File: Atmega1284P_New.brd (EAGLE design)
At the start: 69.5 x 53.3 mm, 28 parts, among them U3 ESP-WROOM-32

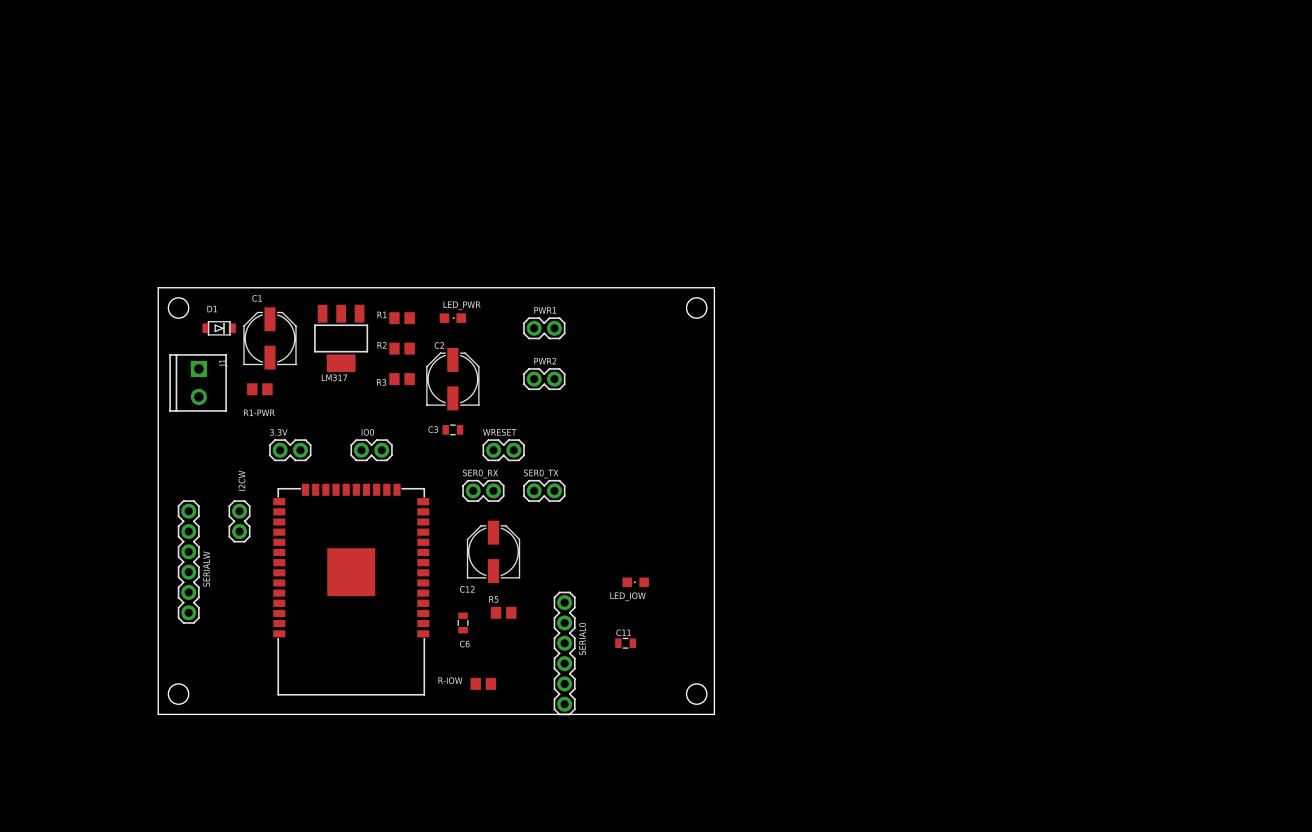
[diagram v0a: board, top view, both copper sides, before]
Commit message: Working Copy
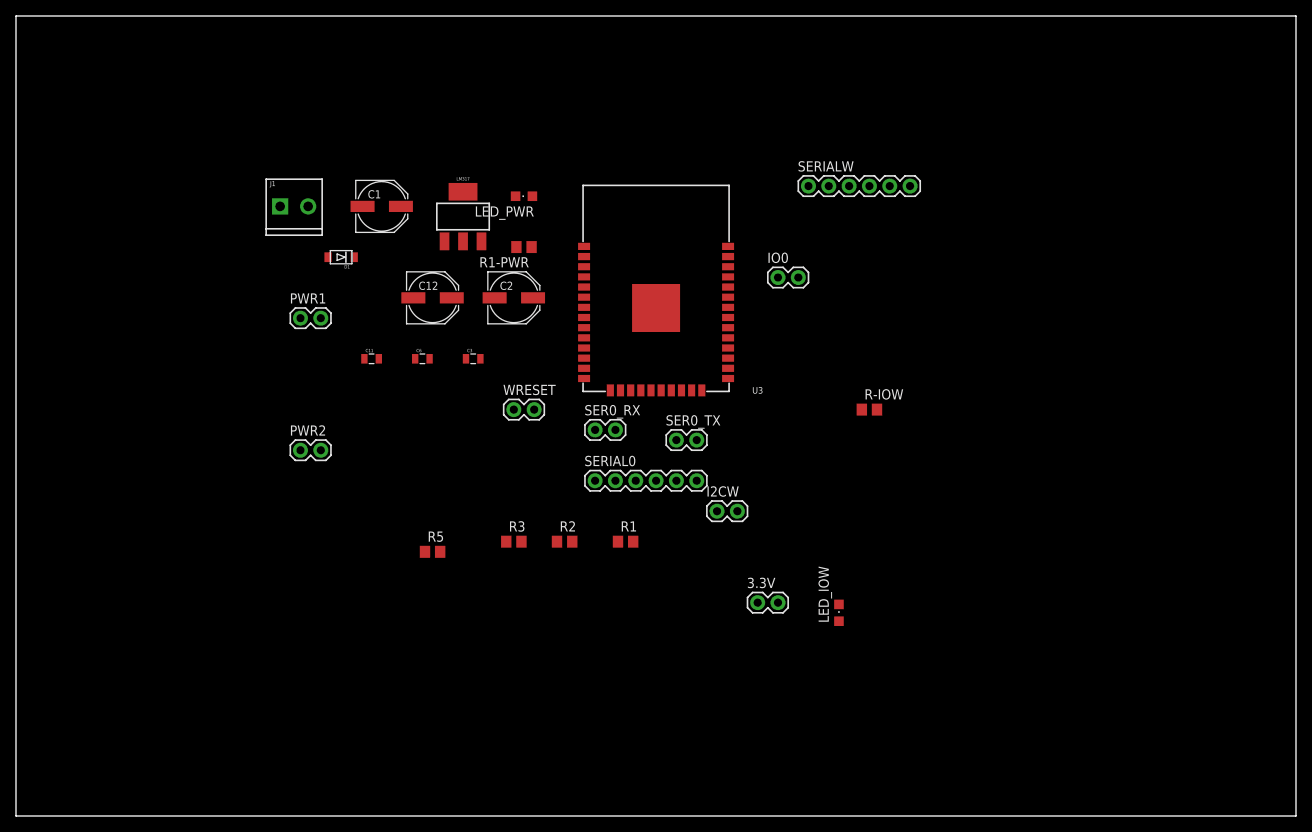
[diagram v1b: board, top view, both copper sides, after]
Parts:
- moved SERIALW 87.5 mm to (99.1, 78.7), turned to 0 degrees
- moved 3.3V 62.7 mm to (92.7, 26.7)
- moved I2CW 59.7 mm to (87.6, 38.1), turned to 0 degrees
- moved R-IOW 59.2 mm to (106.7, 50.8)
- moved IO0 56.4 mm to (95.2, 67.3)
- moved U3 50.4 mm to (80.0, 63.5), turned to 90 degrees
- moved C11 47.7 mm to (44.5, 57.1), turned to 0 degrees
- moved R1 39.5 mm to (76.2, 34.3)
- moved R1-PWR 37.5 mm to (63.5, 71.1)
- moved C6 33.4 mm to (50.8, 57.1), turned to 0 degrees
- moved C12 32.7 mm to (52.1, 64.8), turned to 0 degrees
- moved R2 31.5 mm to (68.6, 34.3)
- moved PWR2 30.5 mm to (35.6, 45.7)
- moved PWR1 29.2 mm to (35.6, 62.2)
- moved LED_IOW 25.7 mm to (102.9, 25.4), turned to 0 degrees
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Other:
- board size 69.5 x 53.3 mm -> 160 x 100 mm
